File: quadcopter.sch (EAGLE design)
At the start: 69 parts, among them J1 AVR_SPI_PRG_6NS, Q1 2.6A, Q2 2.6A, Q3 2.6A, Q4 2.6A, U1 ATMEGA128RFA1, U2 IMU_LSM9DS1TR, Y1 16MHz

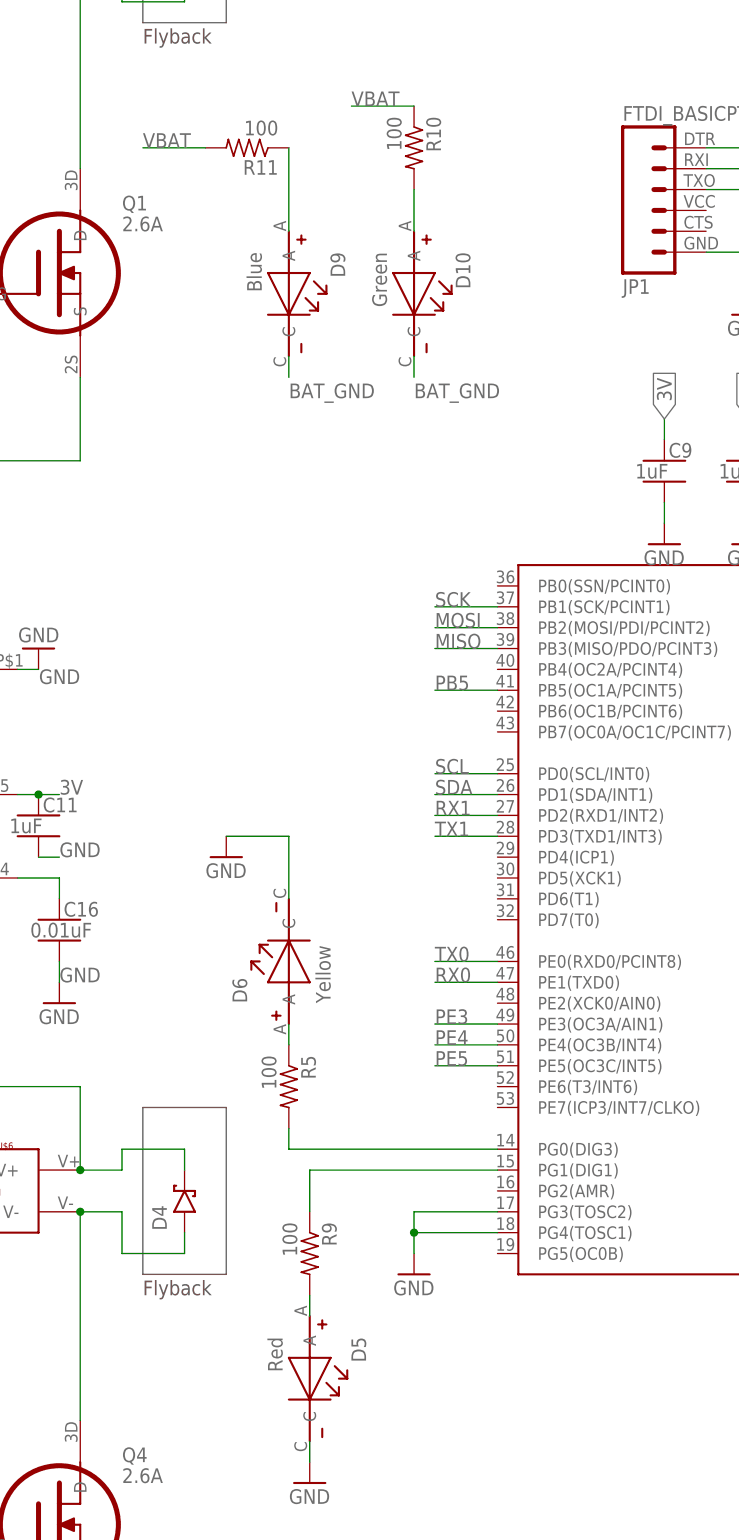
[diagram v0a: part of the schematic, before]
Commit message: Fixed board errors
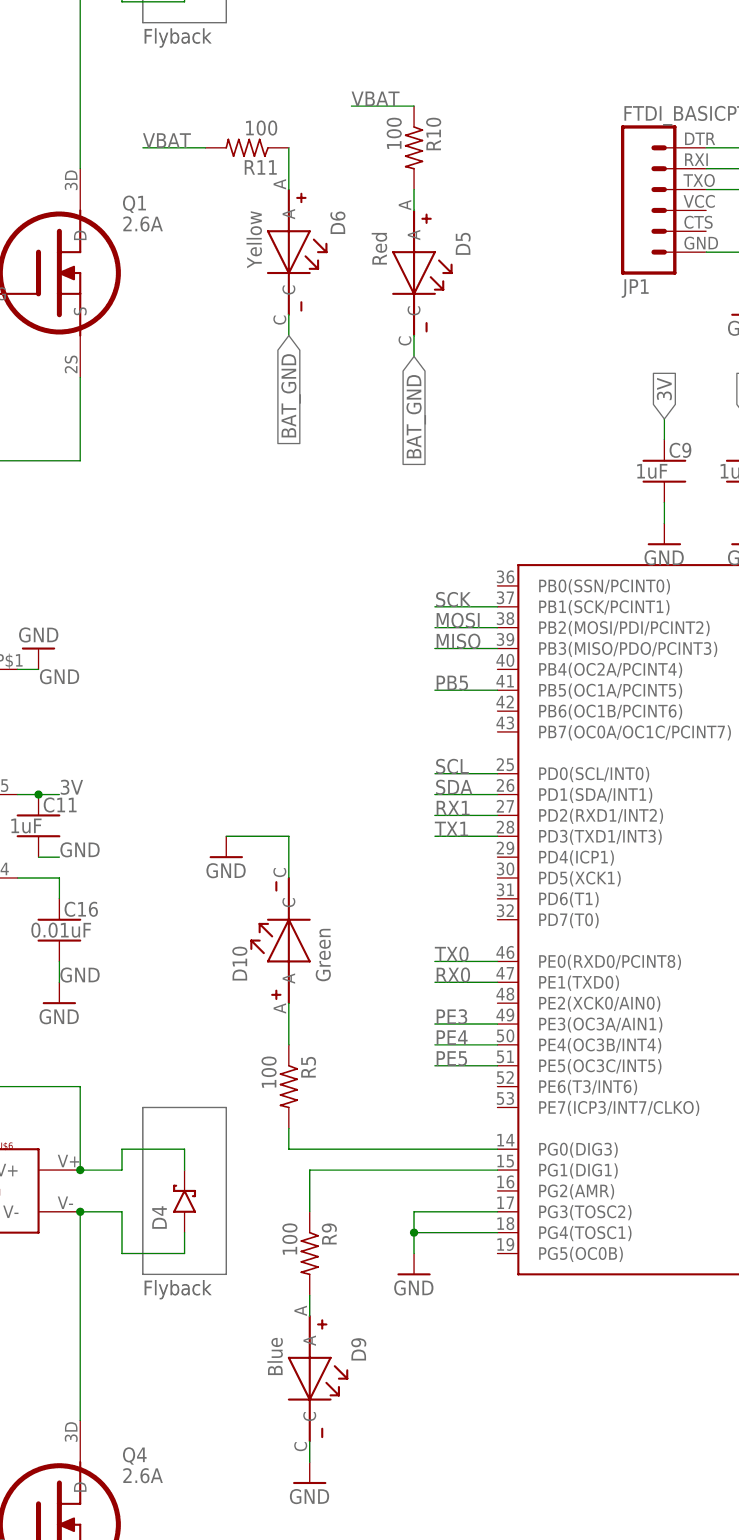
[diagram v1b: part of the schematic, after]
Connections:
- net BAT_GND: now also D5.C, D6.C; no longer D10.C, D9.C
- net GND: now also D10.C, D9.C; no longer D5.C, D6.C
- net N$18: now also D9.A, R9.2; no longer D10.A, R10.2
- net N$19: now also D10.A, R5.1; no longer D5.A, R9.2
- net N$27: now also D5.A, R10.2; no longer D9.A, R11.1
- net N$28: now also R11.1; no longer R5.1
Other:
- moved on the sheet: D10, D5, D6, D9
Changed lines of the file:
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@@
 <instance part="GND23" gate="1" x="99.06" y="-127"/>
 <instance part="J3" gate="G$1" x="78.74" y="-25.4"/>
-<instance part="D9" gate="G$1" x="-109.22" y="60.96" rot="R270"/>
-<instance part="D10" gate="G$1" x="-93.98" y="60.96" rot="R270"/>
-<instance part="D5" gate="G$1" x="-106.68" y="-71.12" rot="R270"/>
-<instance part="D6" gate="G$1" x="-109.22" y="-20.32" rot="R90"/>
+<instance part="D9" gate="G$1" x="-106.68" y="-71.12" rot="R270"/>
+<instance part="D10" gate="G$1" x="-109.22" y="-17.78" rot="R90"/>
+<instance part="D5" gate="G$1" x="-93.98" y="63.5" rot="R270"/>
+<instance part="D6" gate="G$1" x="-109.22" y="66.04" rot="R270"/>
 <instance part="GND24" gate="1" x="-106.68" y="-83.82"/>
 <instance part="GND25" gate="1" x="-116.84" y="-7.62"/>
@@
 </segment>
 <segment>
-<pinref part="D5" gate="G$1" pin="C"/>
-<wire x1="-106.68" y1="-78.74" x2="-106.68" y2="-81.28" width="0.1524" layer="91"/>
-<pinref part="GND24" gate="1" pin="GND"/>
-</segment>
-<segment>
 <pinref part="GND21" gate="1" pin="GND"/>
 <pinref part="C23" gate="G$1" pin="2"/>
@@
 <segment>
 <pinref part="GND25" gate="1" pin="GND"/>
-<pinref part="D6" gate="G$1" pin="C"/>
 <wire x1="-116.84" y1="-5.08" x2="-109.22" y2="-5.08" width="0.1524" layer="91"/>
-<wire x1="-109.22" y1="-5.08" x2="-109.22" y2="-12.7" width="0.1524" layer="91"/>
+<pinref part="D10" gate="G$1" pin="C"/>
+<wire x1="-109.22" y1="-5.08" x2="-109.22" y2="-10.16" width="0.1524" layer="91"/>
 </segment>
 <segment>
@@
 <pinref part="C24" gate="G$1" pin="2"/>
 <wire x1="-53.34" y1="33.02" x2="-53.34" y2="35.56" width="0.1524" layer="91"/>
+</segment>
+<segment>
+<pinref part="D9" gate="G$1" pin="C"/>
+<pinref part="GND24" gate="1" pin="GND"/>
+<wire x1="-106.68" y1="-78.74" x2="-106.68" y2="-81.28" width="0.1524" layer="91"/>
 </segment>
 </net>
@@
 </segment>
 <segment>
-<pinref part="D9" gate="G$1" pin="C"/>
-<wire x1="-109.22" y1="53.34" x2="-109.22" y2="50.8" width="0.1524" layer="91"/>
-<label x="-109.22" y="48.26" size="1.778" layer="95"/>
-</segment>
-<segment>
-<pinref part="D10" gate="G$1" pin="C"/>
-<wire x1="-93.98" y1="53.34" x2="-93.98" y2="50.8" width="0.1524" layer="91"/>
-<label x="-93.98" y="48.26" size="1.778" layer="95"/>
-</segment>
-<segment>
 <pinref part="C10" gate="G$1" pin="2"/>
 <wire x1="-182.88" y1="-7.62" x2="-182.88" y2="-10.16" width="0.1524" layer="91"/>
 <label x="-185.42" y="-12.7" size="1.778" layer="95"/>
+</segment>
+<segment>
+<pinref part="D6" gate="G$1" pin="C"/>
+<wire x1="-109.22" y1="58.42" x2="-109.22" y2="55.88" width="0.1524" layer="91"/>
+<label x="-109.22" y="55.88" size="1.778" layer="95" rot="R270" xref="yes"/>
+</segment>
+<segment>
+<pinref part="D5" gate="G$1" pin="C"/>
+<wire x1="-93.98" y1="55.88" x2="-93.98" y2="53.34" width="0.1524" layer="91"/>
+<label x="-93.98" y="53.34" size="1.778" layer="95" rot="R270" xref="yes"/>
 </segment>
 </net>
@@
 </segment>
 </net>
-<net name="N$27" class="0">
-<segment>
-<pinref part="D9" gate="G$1" pin="A"/>
-<wire x1="-109.22" y1="78.74" x2="-109.22" y2="68.58" width="0.1524" layer="91"/>
-<pinref part="R11" gate="G$1" pin="1"/>
-</segment>
-</net>
-<net name="N$19" class="0">
-<segment>
-<wire x1="-106.68" y1="-60.96" x2="-106.68" y2="-63.5" width="0.1524" layer="91"/>
-<pinref part="D5" gate="G$1" pin="A"/>
-<pinref part="R9" gate="G$1" pin="2"/>
-</segment>
-</net>
-<net name="N$28" class="0">
-<segment>
-<wire x1="-109.22" y1="-30.48" x2="-109.22" y2="-27.94" width="0.1524" layer="91"/>
-<pinref part="D6" gate="G$1" pin="A"/>
-<pinref part="R5" gate="G$1" pin="1"/>
-</segment>
-</net>
-<net name="N$18" class="0">
-<segment>
-<pinref part="D10" gate="G$1" pin="A"/>
-<wire x1="-93.98" y1="73.66" x2="-93.98" y2="68.58" width="0.1524" layer="91"/>
-<pinref part="R10" gate="G$1" pin="2"/>
-</segment>
-</net>
 <net name="N$23" class="0">
 <segment>
@@
 </segment>
 </net>
+<net name="N$18" class="0">
+<segment>
+<pinref part="R9" gate="G$1" pin="2"/>
+<pinref part="D9" gate="G$1" pin="A"/>
+<wire x1="-106.68" y1="-60.96" x2="-106.68" y2="-63.5" width="0.1524" layer="91"/>
+</segment>
+</net>
+<net name="N$19" class="0">
+<segment>
+<pinref part="D10" gate="G$1" pin="A"/>
+<pinref part="R5" gate="G$1" pin="1"/>
+<wire x1="-109.22" y1="-25.4" x2="-109.22" y2="-30.48" width="0.1524" layer="91"/>
+</segment>
+</net>
+<net name="N$27" class="0">
+<segment>
+<pinref part="R10" gate="G$1" pin="2"/>
+<pinref part="D5" gate="G$1" pin="A"/>
+<wire x1="-93.98" y1="73.66" x2="-93.98" y2="71.12" width="0.1524" layer="91"/>
+</segment>
+</net>
+<net name="N$28" class="0">
+<segment>
+<pinref part="R11" gate="G$1" pin="1"/>
+<pinref part="D6" gate="G$1" pin="A"/>
+<wire x1="-109.22" y1="78.74" x2="-109.22" y2="73.66" width="0.1524" layer="91"/>
+</segment>
+</net>

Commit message: Board ready for final review
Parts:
- removed D10: Green, LEDs:LED_OVS5MXBCR4GREEN
- removed D9: Blue, LEDs:LED_OVS5MXBCR4BLUE
- removed R11, R5: 100, quadparts_prebuilt:RESISTOR_SMD-2012-0805-100
- added Q5, Q6: 2.6A, quadparts_connie:N_MOSFET_SI2302CDS_T1_E3
- added SW1: PUSHBUTTON_SMD-VERTICAL, quadparts_prebuilt:PUSHBUTTON_SMD-VERTICAL
- D1, D2, D3, D4: value (none) -> 360mV; device quadparts_prebuilt:DIODE-SCHOTTKY_SMD-SOD123 -> quadparts_prebuilt:DIODE-SCHOTTKY_SMD-SOD123-360MV
- R10, R9: value 100 -> 11; device quadparts_prebuilt:RESISTOR_SMD-2012-0805-100 -> quadparts_prebuilt:RESISTOR_SMD-2012-0805-11
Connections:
- removed net N$11: J1.3
- removed net N$12: J1.5
- removed net N$18: D9.A, R9.2
- removed net N$19: D10.A, R5.1
- removed net N$20: R5.2, U1.PG0(DIG3)
- removed net N$26: R9.1, U1.PG1(DIG1)
- removed net N$28: D6.A, R11.1
- removed net N$6 (its old number): JP2.2
- removed net N$7: JP2.3
- removed net N$8: J1.1
- removed net N$9: J1.4
- new net PB6: Q5.G, U1.PB6(OC1B/PCINT6)
- new net PB7: Q6.G, U1.PB7(OC0A/OC1C/PCINT7)
- net BAT_GND: now also Q5.S, Q6.S; no longer D5.C, D6.C
- net GND: now also SW1.2; no longer D10.C, D9.C
- net MISO: now also J1.1
- net MOSI: now also J1.4
- net N$2: now also D6.C, Q5.D; no longer JP1.3
- net N$3: now also D6.A, R9.2; no longer JP1.2
- net N$4: now also D5.C, Q6.D; no longer C1.2
- net RESET: now also C1.2, J1.5, SW1.1
- net RX0: now also JP1.3
- net RX1: now also JP2.3
- net SCK: now also J1.3
- net TX0: now also JP1.2
- net TX1: now also JP2.2
- net VBAT: now also R9.1; no longer R11.2
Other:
- note added: "LEDs"
- note added: "Motor Drivers"
- note added: "Power"
- note added: "Reset Button"
- moved on the sheet: BATT1, C1, C10, C11, C16, C17, C2, C4, C5, C7, C8, D1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
